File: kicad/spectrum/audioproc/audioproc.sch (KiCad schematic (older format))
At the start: 5 parts

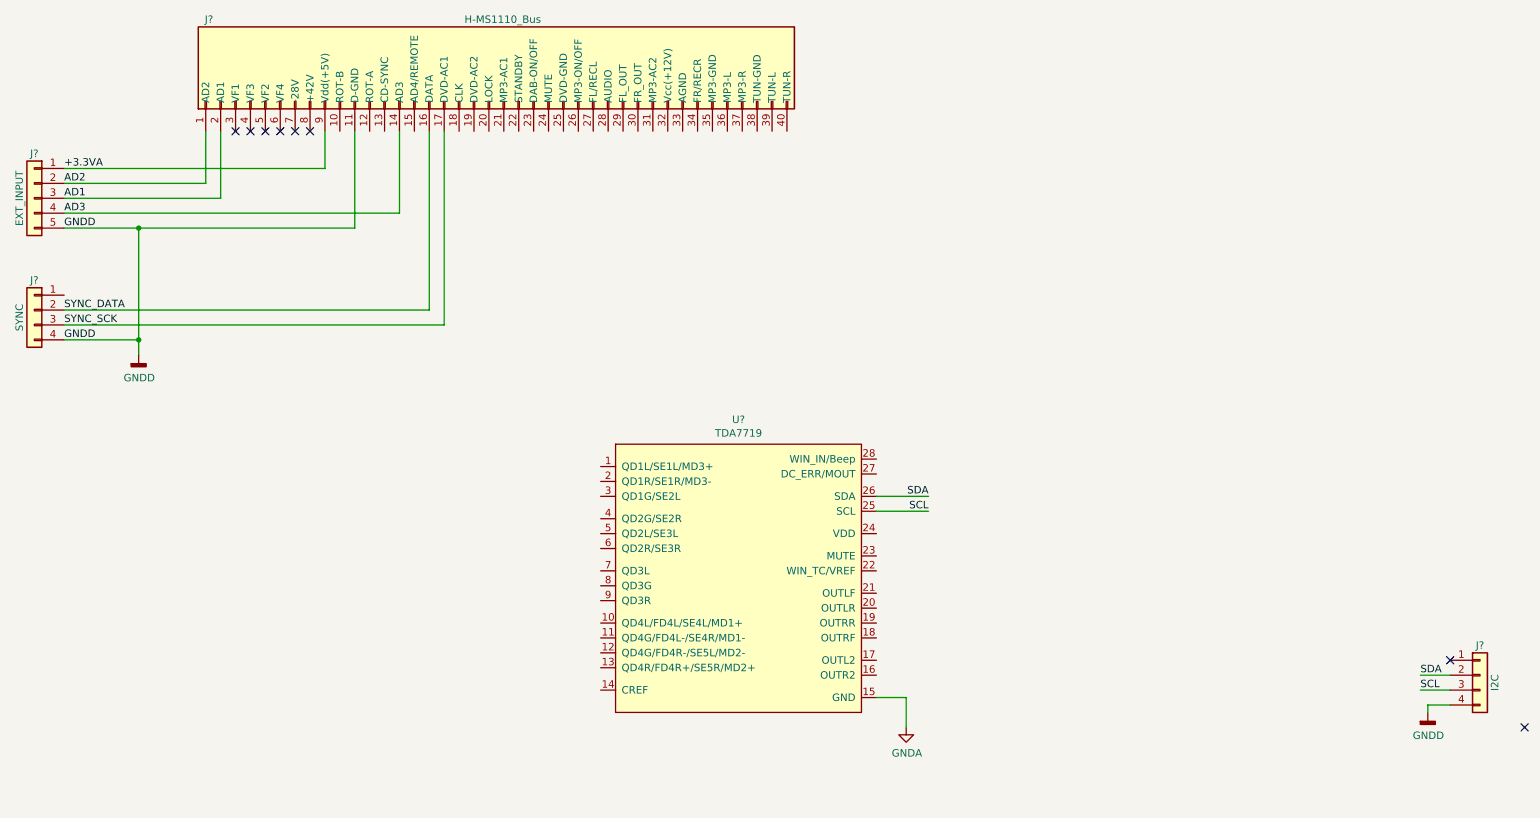
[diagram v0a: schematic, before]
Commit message: Schematics update
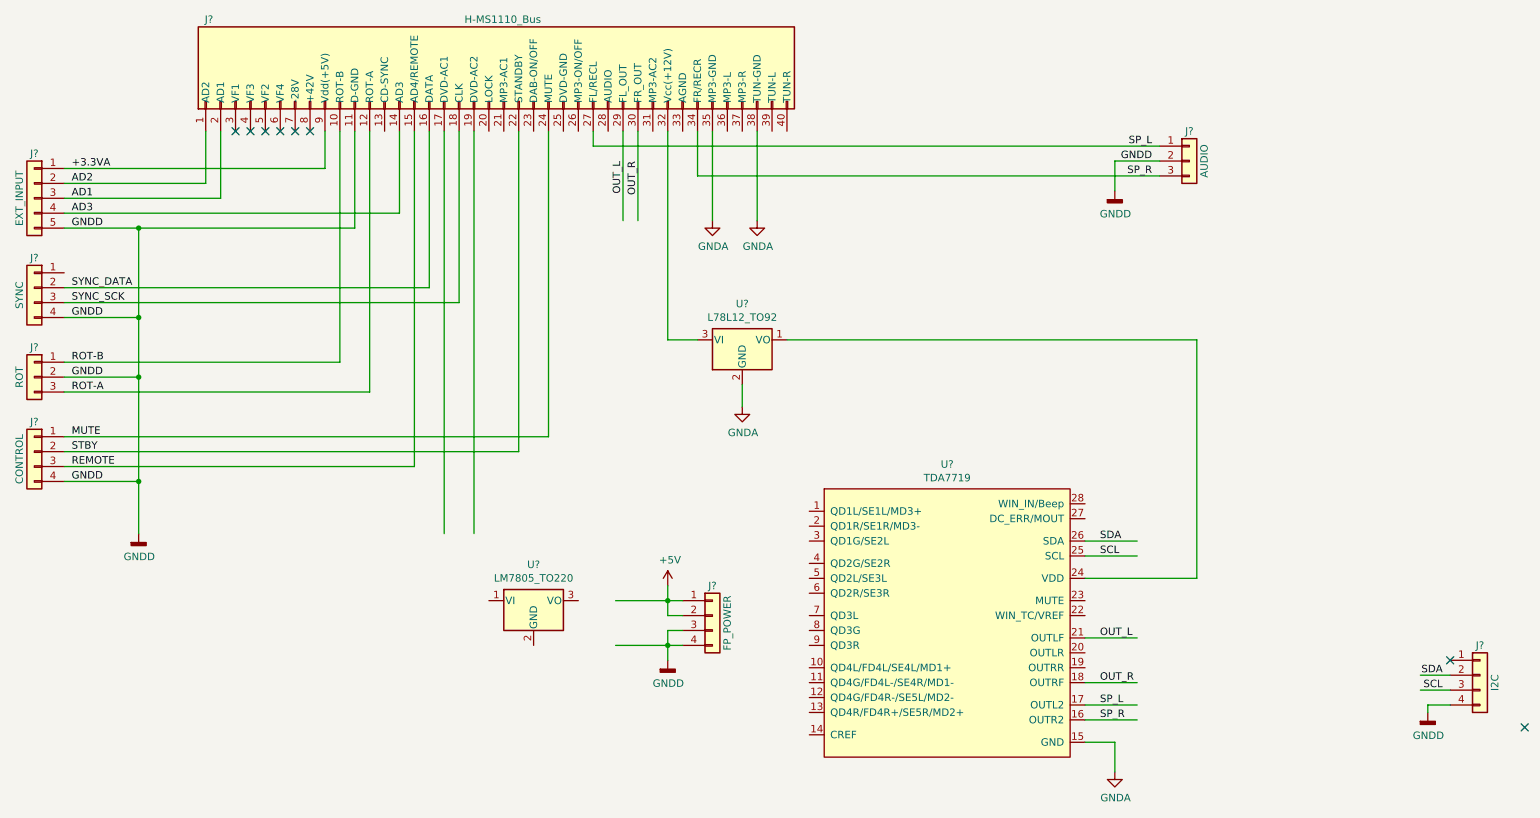
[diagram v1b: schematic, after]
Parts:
- added J?: ROT, symbol Connector_Generic:Conn_01x03
- added J?: CONTROL, Connector_JST:JST_EH_B4B-EH-A_1x04_P2.50mm_Vertical, symbol Connector_Generic:Conn_01x04
- added J?: AUDIO, symbol Connector_Generic:Conn_01x03
- added J?: FP_POWER, Connector_JST:JST_EH_B4B-EH-A_1x04_P2.50mm_Vertical, symbol Connector_Generic:Conn_01x04
- added U?: L78L12_TO92, Package_TO_SOT_THT:TO-92_Inline, symbol Regulator_Linear:L78L12_TO92
- added U?: LM7805_TO220, Package_TO_SOT_THT:TO-220-3_Vertical, symbol Regulator_Linear:LM7805_TO220
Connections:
- net labels added: +5V, MUTE, OUT_L, OUT_R, REMOTE, ROT-A, ROT-B, SP_L, SP_R, STBY
- wire segments 26 -> 72
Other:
- moved on the sheet: J?, U?
